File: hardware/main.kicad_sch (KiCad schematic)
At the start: 10 parts

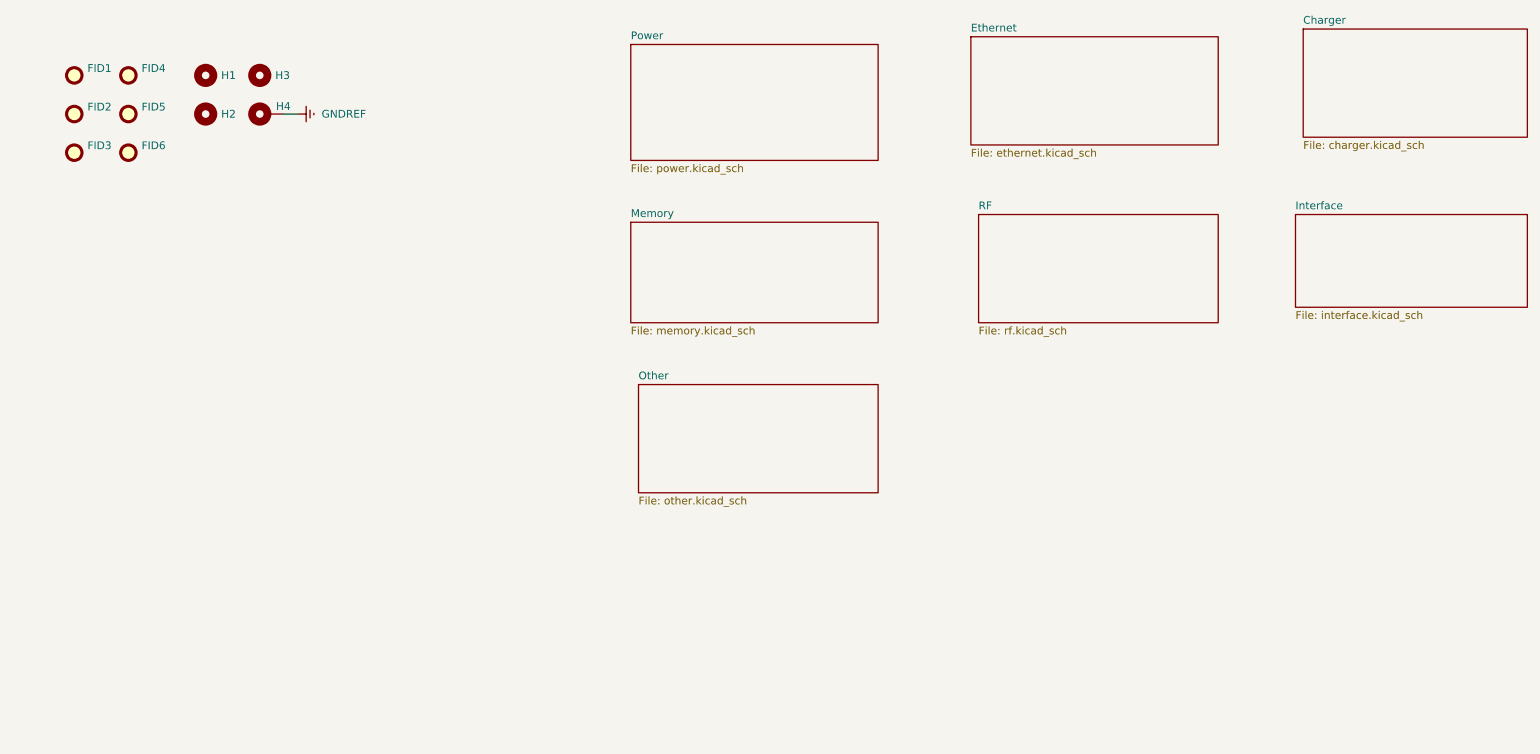
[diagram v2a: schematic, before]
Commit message: update cap and dru
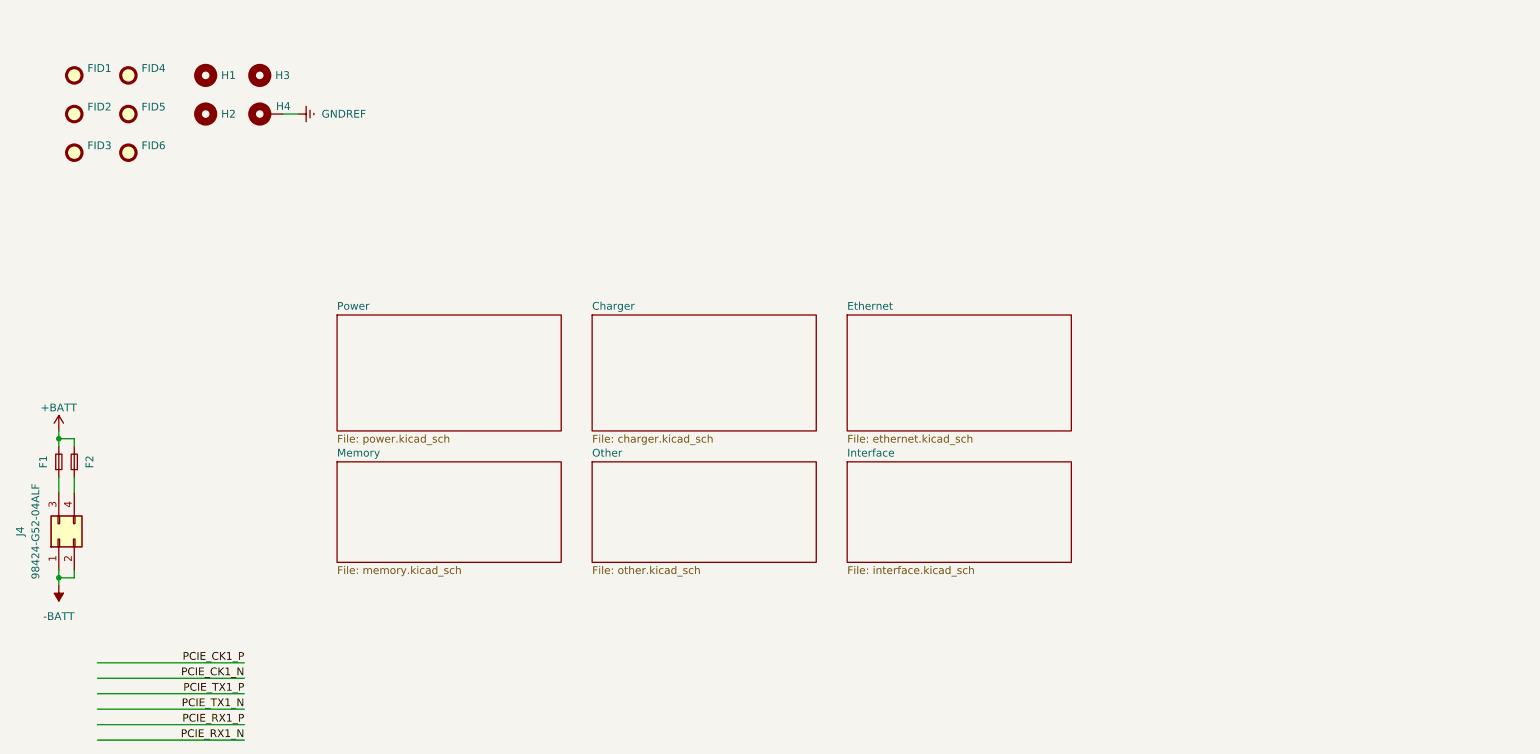
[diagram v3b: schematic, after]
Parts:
- added F1, F2: 12T.30000063AG12S1B02, Fuse:Fuse_1206_3216Metric, symbol Device:Fuse_Small
- added J4: 98424-G52-04ALF, MAS_Package_std:PinSocket_2x02_P2.00mm_Vertical_SMD, symbol Connector_Generic:Conn_02x02_Top_Bottom
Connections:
- new net: F1.1, J4.3 (Pin_3)
- new net: F2.1, J4.4 (Pin_4)
- new net +BATT: F1.2, F2.2
- new net -BATT: J4.1 (Pin_1), J4.2 (Pin_2)
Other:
- removed sheet RF
